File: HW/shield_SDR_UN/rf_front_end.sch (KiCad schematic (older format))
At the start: 92 parts, among them P1 GSG-RF-CONN, P2 GSG-RF-CONN, Q1 MOSFET_P, T1 BALUN, T2 BALUN, U1 MAX2830, U2 SI5351C, U3 MAX5864, X1 GSG-XTAL4PIN

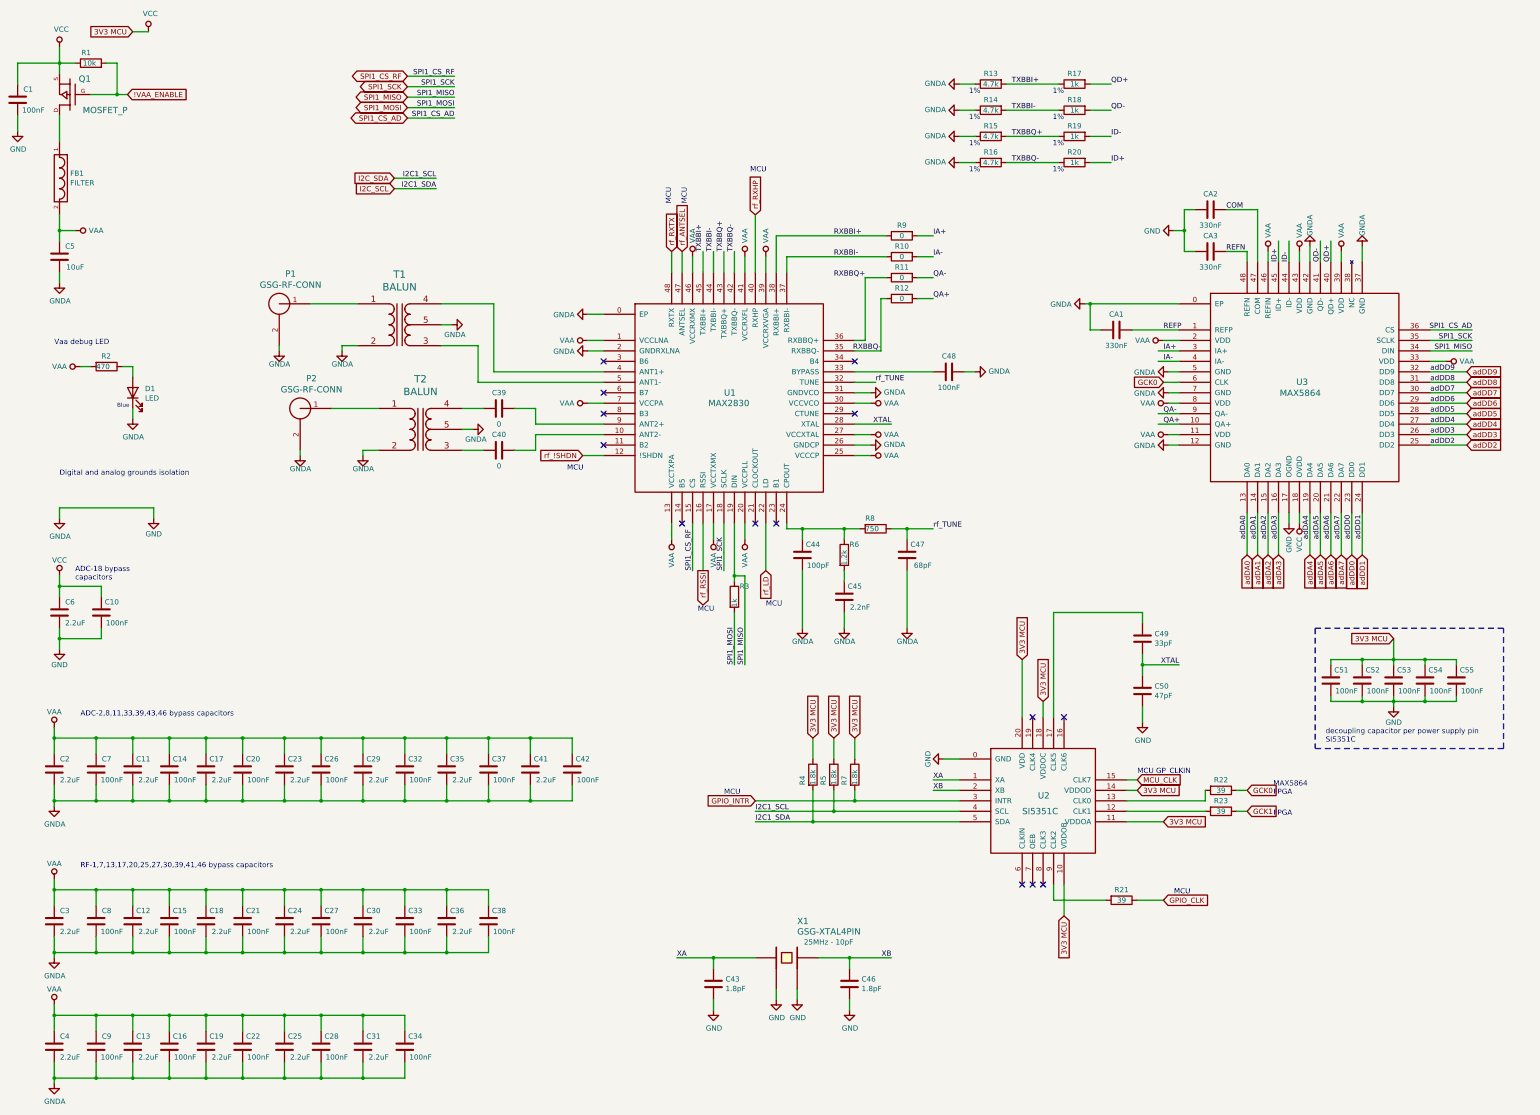
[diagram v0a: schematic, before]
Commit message: organizacion PCB
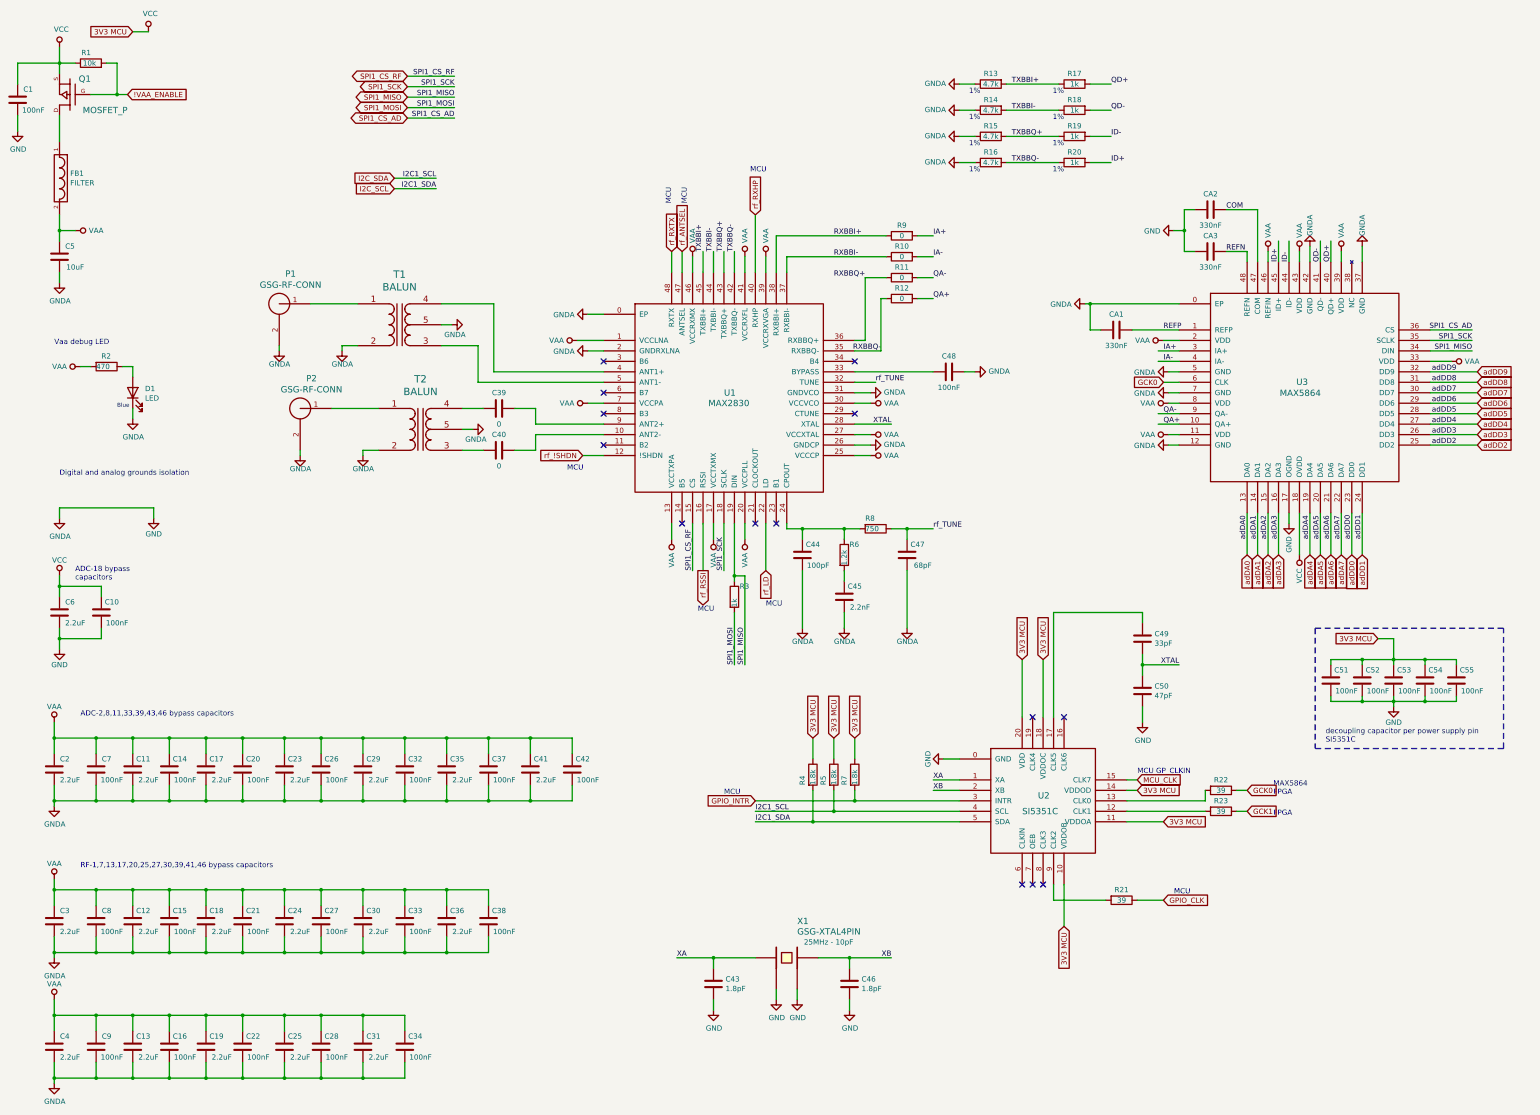
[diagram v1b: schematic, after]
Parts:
- Q1: footprint DMP2305U-7:SOT103P240X110-3N -> lib:SOT103P240X110-3N
- U1: footprint FP-MAX2830:MAX2830ETM&plus_ -> lib:MAX2830ETM&plus_
- U2: footprint QFN50P300X300X60-21N:QFN50P300X300X60-21N -> lib:QFN50P300X300X60-21N
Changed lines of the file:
@@
 Text Label 11800 3650 0    50   ~ 0
 REFP
-Text Label 14350 4050 0    50   ~ 0
+Text Label 14600 4050 2    50   ~ 0
 adDD9
-Text Label 14350 4150 0    50   ~ 0
+Text Label 14600 4150 2    50   ~ 0
 adDD8
-Text Label 14350 4250 0    50   ~ 0
+Text Label 14600 4250 2    50   ~ 0
 adDD7
-Text Label 14350 4350 0    50   ~ 0
+Text Label 14600 4350 2    50   ~ 0
 adDD6
-Text Label 14350 4450 0    50   ~ 0
+Text Label 14600 4450 2    50   ~ 0
 adDD5
-Text Label 14350 4550 0    50   ~ 0
+Text Label 14600 4550 2    50   ~ 0
 adDD4
-Text Label 14350 4650 0    50   ~ 0
+Text Label 14600 4650 2    50   ~ 0
 adDD3
-Text Label 14350 4750 0    50   ~ 0
+Text Label 14600 4750 2    50   ~ 0
 adDD2
 Text Label 13700 5650 1    50   ~ 0
@@
 QA+
 Wire Wire Line
-	13600 5400 13600 5800
-Wire Wire Line
 	13700 5400 13700 5800
-Wire Wire Line
-	14350 4050 14700 4050
-Wire Wire Line
-	14350 4150 14700 4150
-Wire Wire Line
-	14350 4250 14700 4250
-Wire Wire Line
-	14350 4350 14700 4350
-Wire Wire Line
-	14350 4450 14700 4450
-Wire Wire Line
-	14350 4550 14700 4550
-Wire Wire Line
-	14350 4650 14700 4650
-Wire Wire Line
-	14350 4750 14700 4750
-Text GLabel 14700 4050 2    50   Input ~ 0
+Text GLabel 14800 4050 2    50   Input ~ 0
 adDD9
-Text GLabel 14700 4150 2    50   Input ~ 0
+Text GLabel 14800 4150 2    50   Input ~ 0
 adDD8
-Text GLabel 14700 4250 2    50   Input ~ 0
+Text GLabel 14800 4250 2    50   Input ~ 0
 adDD7
-Text GLabel 14700 4350 2    50   Input ~ 0
+Text GLabel 14800 4350 2    50   Input ~ 0
 adDD6
-Text GLabel 14700 4450 2    50   Input ~ 0
+Text GLabel 14800 4450 2    50   Input ~ 0
 adDD5
-Text GLabel 14700 4550 2    50   Input ~ 0
+Text GLabel 14800 4550 2    50   Input ~ 0
 adDD4
-Text GLabel 14700 4650 2    50   Input ~ 0
+Text GLabel 14800 4650 2    50   Input ~ 0
 adDD3
-Text GLabel 14700 4750 2    50   Input ~ 0
+Text GLabel 14800 4750 2    50   Input ~ 0
 adDD2
 Text GLabel 13700 5800 3    50   Input ~ 0
@@
 adDA0
 Wire Wire Line
-	12800 2900 12800 3000
-Wire Wire Line
 	13100 2900 13100 3000
 Wire Wire Line
@@
 L power:VAA #PWR069
 U 1 1 5CCBDAAC
-P 14500 3950
-F 0 "#PWR069" H 14500 3800 50  0001 C CNN
-F 1 "VAA" V 14500 4150 50  0000 C CNN
-F 2 "" H 14500 3950 50  0001 C CNN
-F 3 "" H 14500 3950 50  0001 C CNN
-	1    14500 3950
+P 14550 3950
+F 0 "#PWR069" H 14550 3800 50  0001 C CNN
+F 1 "VAA" V 14550 4150 50  0000 C CNN
+F 2 "" H 14550 3950 50  0001 C CNN
+F 3 "" H 14550 3950 50  0001 C CNN
+	1    14550 3950
 	0    1    1    0
 $EndComp
-Wire Wire Line
-	14500 3950 14350 3950
 $Comp
 L power:VAA #PWR057
@@
 F 0 "Q1" H 1150 1250 60  0000 L CNN
 F 1 "MOSFET_P" H 800 1550 60  0000 L CNN
-F 2 "DMP2305U-7:SOT103P240X110-3N" H 1350 1400 60  0001 C CNN
+F 2 "lib:SOT103P240X110-3N" H 1350 1400 60  0001 C CNN
 F 3 "https://www.diodes.com/assets/Datasheets/ds31737.pdf" H 1350 1400 60  0001 C CNN
 F 4 "DMP2305UDICT-ND" H 1350 1400 50  0001 C CNN "Digikey"
@@
 	1250 3200 1250 3100
 $Comp
-L power:VCC #PWR064
-U 1 1 5CD923B4
-P 13100 5500
-F 0 "#PWR064" H 13100 5350 50  0001 C CNN
-F 1 "VCC" V 13100 5700 50  0000 C CNN
-F 2 "" H 13100 5500 50  0001 C CNN
-F 3 "" H 13100 5500 50  0001 C CNN
-	1    13100 5500
-	-1   0    0    1
-$EndComp
-Wire Wire Line
-	13100 5500 13100 5400
-$Comp
 L Device:C C5
 U 1 1 5CD06356
@@
 L power:VAA #PWR02
 U 1 1 5CDED280
-P 1200 7450
-F 0 "#PWR02" H 1200 7300 50  0001 C CNN
-F 1 "VAA" H 1200 7600 50  0000 C CNN
-F 2 "" H 1200 7450 50  0001 C CNN
-F 3 "" H 1200 7450 50  0001 C CNN
-	1    1200 7450
+P 1200 7400
+F 0 "#PWR02" H 1200 7250 50  0001 C CNN
+F 1 "VAA" H 1200 7550 50  0000 C CNN
+F 2 "" H 1200 7400 50  0001 C CNN
+F 3 "" H 1200 7400 50  0001 C CNN
+	1    1200 7400
 	1    0    0    -1
 $EndComp
@@
 	1200 8200 1200 8150
 Wire Wire Line
-	1200 7450 1200 7550
-Wire Wire Line
 	1600 7700 1600 7550
 Wire Wire Line
 	1600 7550 1200 7550
-Connection ~ 1200 7550
 Wire Wire Line
 	1200 7550 1200 7700
@@
 F 0 "U1" H 7600 4350 60  0000 L CNN
 F 1 "MAX2830" H 7450 4250 60  0000 L CNN
-F 2 "FP-MAX2830:MAX2830ETM&plus_" H 7650 4300 60  0001 C CNN
+F 2 "lib:MAX2830ETM&plus_" H 7650 4300 60  0001 C CNN
 F 3 "https://datasheets.maximintegrated.com/en/ds/MAX2830.pdf" H 7650 4300 60  0001 C CNN
 F 4 "MAX2830ETM+TCT-ND" H 7650 4300 50  0001 C CNN "Digikey"
@@
 	9000 4750 8850 4750
 $Comp
-L power:VAA #PWR025
-U 1 1 5CDC13A5
-P 6300 3750
-F 0 "#PWR025" H 6300 3600 50  0001 C CNN
-F 1 "VAA" V 6300 3950 50  0000 C CNN
-F 2 "" H 6300 3750 50  0001 C CNN
-F 3 "" H 6300 3750 50  0001 C CNN
-	1    6300 3750
-	0    -1   -1   0
-$EndComp
-$Comp
 L power:VAA #PWR027
 U 1 1 5CDC41DC
@@
 	9000 4350 8850 4350
 Wire Wire Line
-	9000 4650 8850 4650
-Wire Wire Line
 	8850 4850 9000 4850
 Wire Wire Line
@@
 NoConn ~ 10650 8950
 NoConn ~ 10550 8950
-Text GLabel 10850 9250 3    50   Input ~ 0
-3V3 MCU
-Wire Wire Line
-	10850 9250 10850 8950
 Wire Wire Line
 	11250 9100 10750 9100
@@
 Text GLabel 11800 9100 2    50   Input ~ 0
 GPIO_CLK
-Text GLabel 11800 8350 2    50   Input ~ 0
-3V3 MCU
-Wire Wire Line
-	11800 8350 11450 8350
-Text GLabel 10450 6800 1    50   Input ~ 0
-3V3 MCU
 $Comp
 L power:GND #PWR046
@@
 Text Notes 11550 7900 0    50   ~ 0
 MCU GP_CLKIN
-Text GLabel 11550 8050 2    50   Input ~ 0
-3V3 MCU
 Wire Wire Line
 	11550 8050 11450 8050
-Text GLabel 10650 7200 1    50   Input ~ 0
-3V3 MCU
-Wire Wire Line
-	10650 7200 10650 7350
 NoConn ~ 10550 7350
 $Comp
@@
 	1    0    0    -1
 $EndComp
-Text GLabel 8850 7550 1    50   Input ~ 0
-3V3 MCU
-Text GLabel 8650 7550 1    50   Input ~ 0
-3V3 MCU
-Text GLabel 8450 7550 1    50   Input ~ 0
-3V3 MCU
 Wire Wire Line
 	8450 7550 8450 7750
@@
 L power:VAA #PWR06
 U 1 1 5CEC6014
-P 1200 10100
-F 0 "#PWR06" H 1200 9950 50  0001 C CNN
-F 1 "VAA" H 1200 10250 50  0000 C CNN
-F 2 "" H 1200 10100 50  0001 C CNN
-F 3 "" H 1200 10100 50  0001 C CNN
-	1    1200 10100
+P 1200 10050
+F 0 "#PWR06" H 1200 9900 50  0001 C CNN
+F 1 "VAA" H 1200 10200 50  0000 C CNN
+F 2 "" H 1200 10050 50  0001 C CNN
+F 3 "" H 1200 10050 50  0001 C CNN
+	1    1200 10050
 	1    0    0    -1
 $EndComp
@@
 	1200 10850 1200 10800
 Wire Wire Line
-	1200 10100 1200 10200
-Wire Wire Line
 	1600 10350 1600 10200
 Wire Wire Line
 	1600 10200 1200 10200
-Connection ~ 1200 10200
 Wire Wire Line
 	1200 10200 1200 10350
@@
 NoConn ~ 8850 3950
 Wire Wire Line
-	7200 3100 7200 2900
-Wire Wire Line
 	7100 3100 7100 2900
 Text GLabel 7200 2900 1    50   Input ~ 0
@@
 F 0 "U2" H 10600 8200 60  0000 L CNN
 F 1 "SI5351C" H 10450 8050 60  0000 L CNN
-F 2 "QFN50P300X300X60-21N:QFN50P300X300X60-21N" H 10650 8150 60  0001 C CNN
+F 2 "lib:QFN50P300X300X60-21N" H 10650 8150 60  0001 C CNN
 F 3 "https://www.silabs.com/documents/public/data-sheets/Si5351-B.pdf" H 10650 8150 60  0001 C CNN
 F 4 "336-5160-1-ND" H 10650 8150 50  0001 C CNN "Digikey"
@@
 	1    0    0    -1
 $EndComp
-Text GLabel 14000 6600 0    50   Input ~ 0
-3V3 MCU
 Wire Wire Line
 	13400 6850 13400 6800
@@
 	14000 6800 14300 6800
 Wire Wire Line
-	14000 6800 14000 6600
-Wire Wire Line
 	13700 6850 13700 6800
 Connection ~ 13700 6800
@@
 SPI1_SCK
 Wire Wire Line
-	6450 3750 6300 3750
-Wire Wire Line
 	1250 6700 1250 6600
 Connection ~ 1250 6600
 Wire Wire Line
 	2150 5450 2150 5350
+Wire Wire Line
+	9000 4650 8850 4650
+Wire Wire Line
+	12800 2900 12800 3000
+Wire Wire Line
+	11800 8350 11450 8350
+Wire Wire Line
+	7200 2900 7200 3100
+Wire Wire Line
+	14350 4550 14800 4550
+Wire Wire Line
+	14350 4450 14800 4450
+Wire Wire Line
+	14550 3950 14350 3950
+Wire Wire Line
+	1200 7400 1200 7550
+Connection ~ 1200 7550
+$Comp
+L power:VAA #PWR0155
+U 1 1 5CEEB354
+P 6200 3750
+F 0 "#PWR0155" H 6200 3600 50  0001 C CNN
+F 1 "VAA" V 6200 3950 50  0000 C CNN
+F 2 "" H 6200 3750 50  0001 C CNN
+F 3 "" H 6200 3750 50  0001 C CNN
+	1    6200 3750
+	0    -1   -1   0
+$EndComp
+Wire Wire Line
+	6200 3750 6450 3750
+Wire Wire Line
+	1200 10050 1200 10200
+Connection ~ 1200 10200
+$Comp
+L power:VCC #PWR0156
+U 1 1 5CF2950C
+P 13100 5800
+F 0 "#PWR0156" H 13100 5650 50  0001 C CNN
+F 1 "VCC" V 13100 6000 50  0000 C CNN
+F 2 "" H 13100 5800 50  0001 C CNN
+F 3 "" H 13100 5800 50  0001 C CNN
+	1    13100 5800
+	-1   0    0    1
+$EndComp
+Wire Wire Line
+	13100 5400 13100 5800
+Wire Wire Line
+	13600 5400 13600 5800
+Wire Wire Line
+	14350 4650 14800 4650
+Wire Wire Line
+	14350 4350 14800 4350
+Wire Wire Line
+	14350 4250 14800 4250
+Wire Wire Line
+	14350 4150 14800 4150
+Wire Wire Line
+	14350 4050 14800 4050
+Wire Wire Line
+	14350 4750 14800 4750
+Wire Wire Line
+	10650 7350 10650 6800
+Wire Wire Line
+	14000 6800 14000 6600
+Wire Wire Line
+	14000 6600 13850 6600
+Text GLabel 10850 9350 3    50   Input ~ 0
+3V3 MCU
+Wire Wire Line
+	10850 8950 10850 9350
+Text GLabel 11800 8350 2    50   Input ~ 0
+3V3 MCU
+Text GLabel 11550 8050 2    50   Input ~ 0
+3V3 MCU
+Text GLabel 10450 6800 1    50   Input ~ 0
+3V3 MCU
+Text GLabel 10650 6800 1    50   Input ~ 0
+3V3 MCU
+Text GLabel 8450 7550 1    50   Input ~ 0
+3V3 MCU
+Text GLabel 8650 7550 1    50   Input ~ 0
+3V3 MCU
+Text GLabel 8850 7550 1    50   Input ~ 0
+3V3 MCU
+Text GLabel 13850 6600 0    50   Input ~ 0
+3V3 MCU
 $EndSCHEMATC

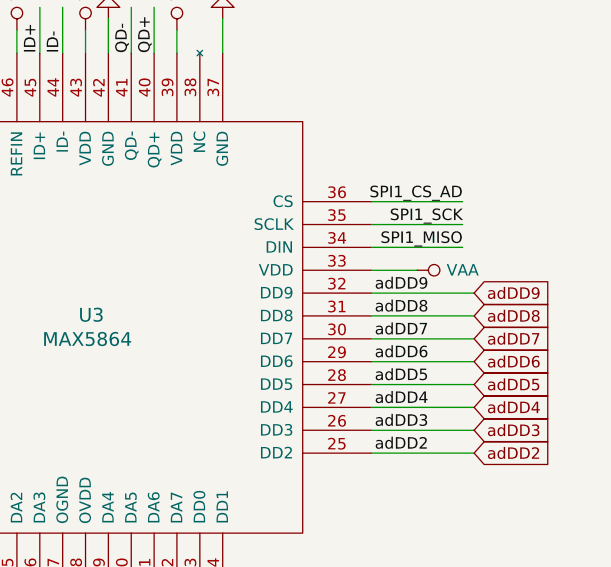
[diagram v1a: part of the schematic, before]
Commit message: Omega 2 PCB
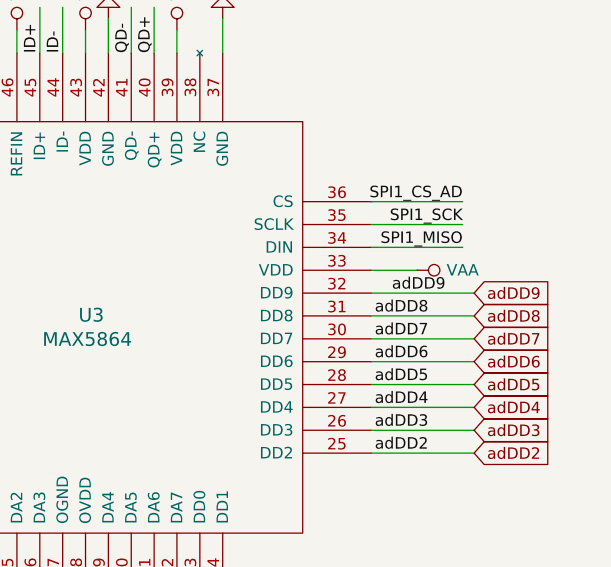
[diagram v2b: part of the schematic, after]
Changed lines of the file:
@@
 Text Label 11800 3650 0    50   ~ 0
 REFP
-Text Label 14600 4050 2    50   ~ 0
+Text Label 14675 4050 2    50   ~ 0
 adDD9
 Text Label 14600 4150 2    50   ~ 0
@@
 $EndComp
 Wire Wire Line
-	7300 2950 7300 3100
-Wire Wire Line
 	7800 2950 7800 3100
 Wire Wire Line
@@
 	14350 4150 14800 4150
 Wire Wire Line
-	14350 4050 14800 4050
-Wire Wire Line
 	14350 4750 14800 4750
 Wire Wire Line
@@
 Text GLabel 13850 6600 0    50   Input ~ 0
 3V3 MCU
+Wire Wire Line
+	14350 4050 14800 4050
+Wire Wire Line
+	7300 2950 7300 3100
 $EndSCHEMATC
